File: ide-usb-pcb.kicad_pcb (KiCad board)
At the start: 2 copper layers, 28 parts, among them J1 Conn_02x20_Odd_Even, J2 STM32F4_Discovery_Header, U1 TXS0108EPW, U2 TXS0108EPW

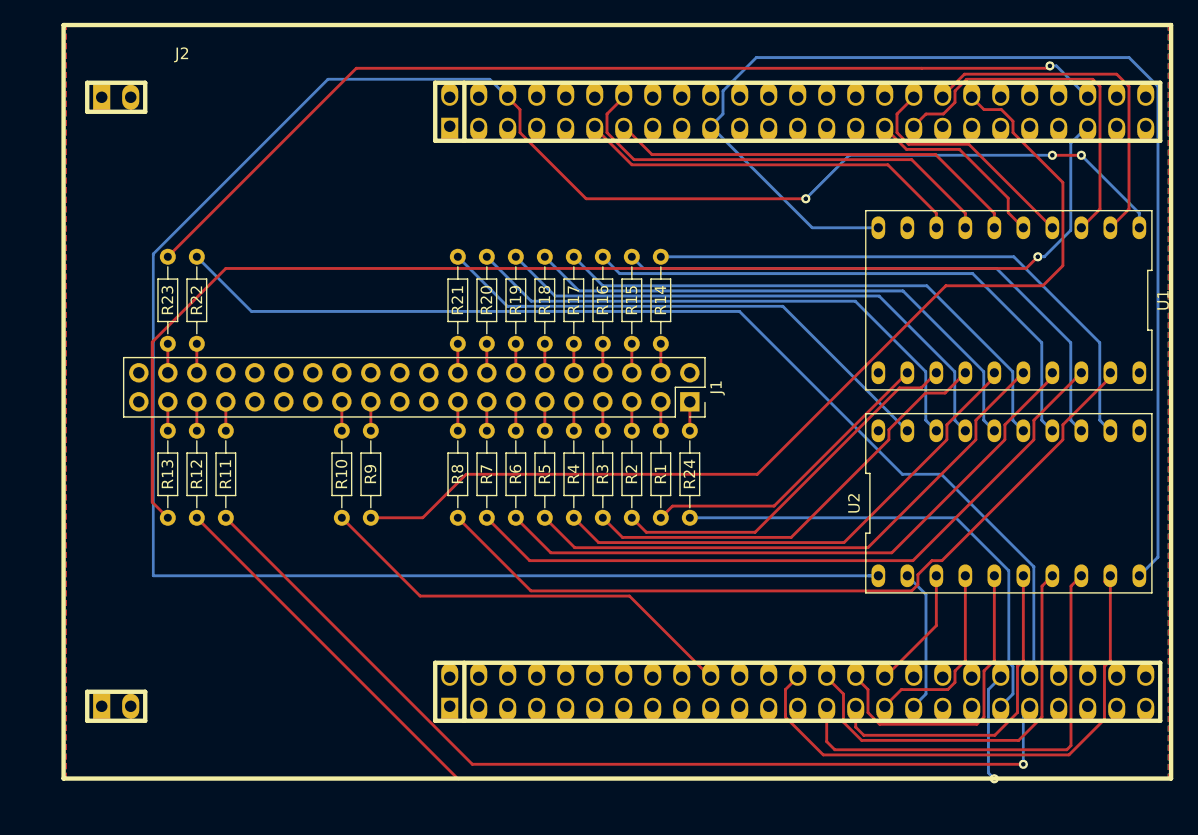
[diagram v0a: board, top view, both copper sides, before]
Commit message: Yet another PCB design
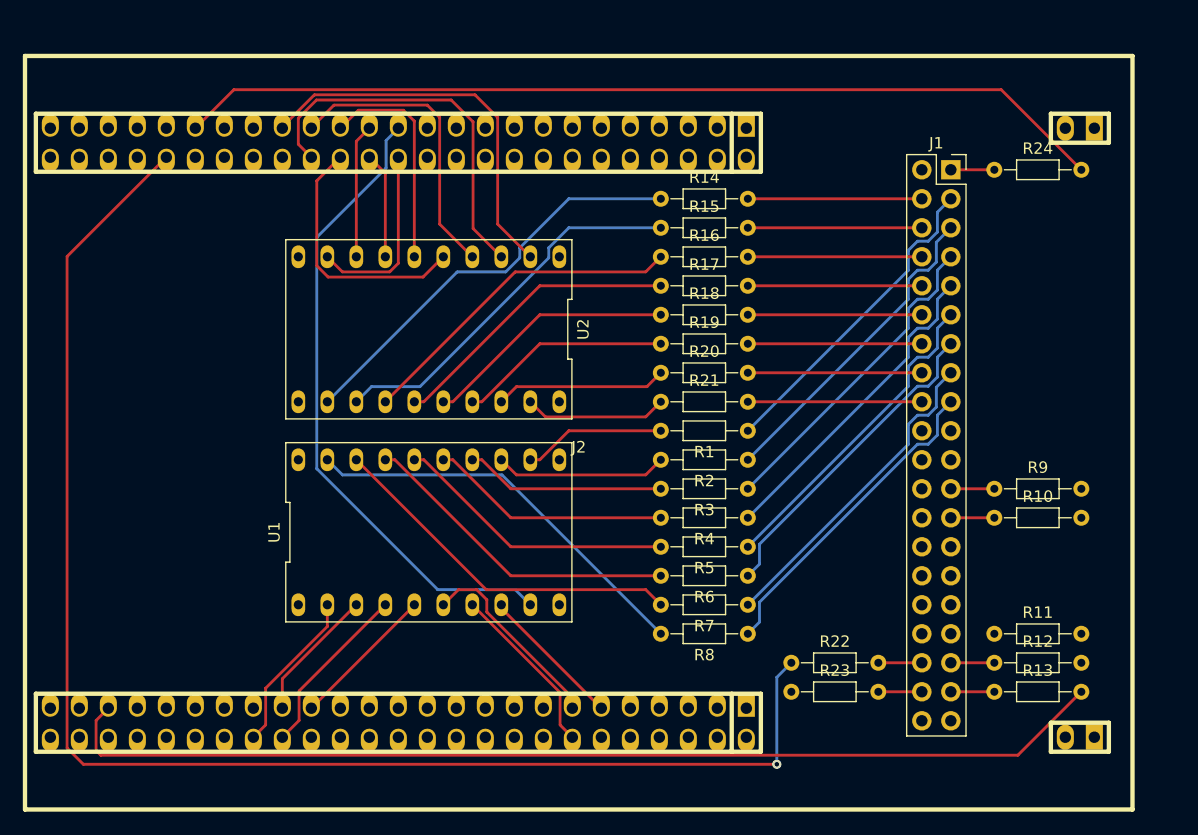
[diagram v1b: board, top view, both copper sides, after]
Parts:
- moved R13 75.9 mm to (118.1, 99.1), turned to 0 degrees
- moved R12 72.7 mm to (118.1, 96.5), turned to 0 degrees
- moved R11 69.6 mm to (118.1, 94.0), turned to 0 degrees
- moved R23 66.6 mm to (100.3, 99.1), turned to 0 degrees
- moved R22 63.1 mm to (100.3, 96.5), turned to 0 degrees
- moved R10 57.7 mm to (118.1, 83.8), turned to 0 degrees
- moved R9 54.8 mm to (118.1, 81.3), turned to 0 degrees
- moved U1 54.7 mm to (68.6, 85.1), turned to 0 degrees
- moved U2 53.0 mm to (68.6, 67.3), turned to 180 degrees
- moved R24 35.1 mm to (118.1, 53.3), turned to 0 degrees
- moved R8 31.0 mm to (96.5, 94.0), turned to 180 degrees
- moved J1 30.6 mm to (114.3, 53.3), turned to 0 degrees
- moved R7 27.5 mm to (96.5, 91.4), turned to 180 degrees
- moved R6 24.0 mm to (96.5, 88.9), turned to 180 degrees
- moved R21 21.8 mm to (88.9, 73.7), turned to 0 degrees
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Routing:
- net +3V3: track 195.7 -> 0.00 mm, vias 3 -> 0
- net /OE: track 105.8 -> 0.00 mm
- net /DA0: track 88.9 -> 0.00 mm, vias 1 -> 0
- net /DIOW: track 88.7 -> 0.00 mm
- net /CS1: track 88.5 -> 0.00 mm, vias 1 -> 0
- net /DA1: track 84.1 -> 0.00 mm, vias 1 -> 0
- net /DD7A: track 0.00 -> 56.4 mm
- net /RESET: track 42.3 -> 81.9 mm
- net /DIOR: track 38.1 -> 0.00 mm
- net /DD0B: track 69.2 -> 35.5 mm
- net /DD15B: track 46.1 -> 12.5 mm
- net /DD14B: track 48.2 -> 15.0 mm
- net /DA2: track 94.4 -> 127.5 mm, vias 0 -> 1
- net /DD8A: track 48.1 -> 16.4 mm
- net /DD13B: track 48.2 -> 18.6 mm
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- removed copper zone on B.Cu, net GND
- removed copper zone on F.Cu, net GND
